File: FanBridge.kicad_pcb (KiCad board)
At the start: 2 copper layers, 15.2 x 10.2 mm, 15 parts, among them P1 CONN_01X01, P2 CONN_01X01, P3 CONN_1, P4 CONN_1, P5 CONN_1, P6 CONN_1, Q1 IRF7309IPBF, Q2 2N7002, Q3 2N7002, Q4 IRF7309IPBF

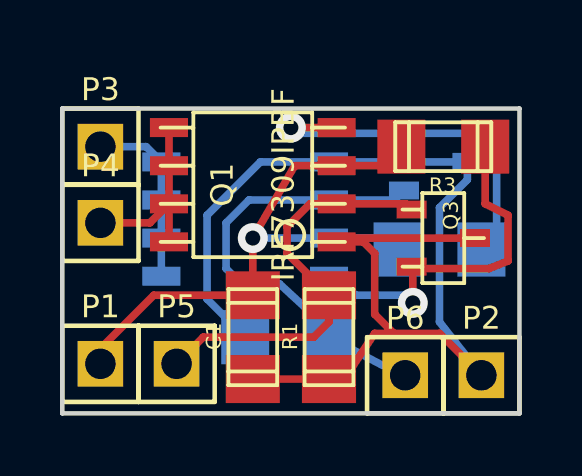
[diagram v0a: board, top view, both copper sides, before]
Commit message: 18.08.2017
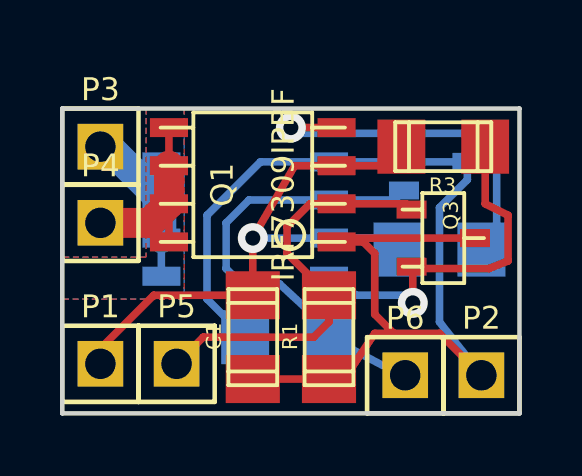
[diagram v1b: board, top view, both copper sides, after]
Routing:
- net /power+: track 6.36 -> 7.63 mm
- net /power-: track 6.05 -> 6.58 mm
- added copper zone on F.Cu, net /power+
- added copper zone on B.Cu, net /power-
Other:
- net class Output added: clearance 0.254, trace_width 1, via_dia 1, via_drill 0.635
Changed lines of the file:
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@@
     (thickness 1.6)
     (drawings 4)
-    (tracks 89)
+    (tracks 90)
     (zones 0)
     (modules 15)
@@
     (last_trace_width 0.254)
     (trace_clearance 0.254)
-    (zone_clearance 0.508)
+    (zone_clearance 0.5)
     (zone_45_only no)
     (trace_min 0.254)
@@
     (pad_to_mask_clearance 0.2)
     (aux_axis_origin 0 0)
-    (visible_elements FFFE5FBF)
+    (visible_elements FFFE7FBF)
     (pcbplotparams
       (layerselection 3178497)
@@
     (uvia_drill 0.127)
     (add_net "")
-    (add_net +8V)
     (add_net /control+)
     (add_net /control-)
+    (add_net N-000004)
+    (add_net N-000005)
+  )
+  (net_class Output ""
+    (clearance 0.254)
+    (trace_width 1)
+    (via_dia 1)
+    (via_drill 0.635)
+    (uvia_dia 0.508)
+    (uvia_drill 0.127)
     (add_net /power+)
     (add_net /power-)
-    (add_net GND)
-    (add_net N-000004)
-    (add_net N-000005)
   )
   (net_class Power ""
@@
     (uvia_dia 0.508)
     (uvia_drill 0.127)
+    (add_net +8V)
+    (add_net GND)
   )
   (module c_1206 (layer F.Cu)
@@
   (gr_line (start 121.92 73.66) (end 121.92 63.5) (angle 90) (layer Edge.Cuts) (width 0.15))
   (gr_line (start 137.16 73.66) (end 121.92 73.66) (angle 90) (layer Edge.Cuts) (width 0.15))
-  (segment (start 128.27 67.818) (end 128.27 69.723) (width 0.254) (layer F.Cu) (net 1) (status 800000))
-  (segment (start 123.19 72.009) (end 123.19 71.501) (width 0.254) (layer F.Cu) (net 1) (status C00000))
-  (segment (start 123.19 71.501) (end 124.968 69.723) (width 0.254) (layer F.Cu) (net 1) (status 400000))
-  (segment (start 124.968 69.723) (end 128.27 69.723) (width 0.254) (layer F.Cu) (net 1) (status 800000))
+  (segment (start 128.27 67.818) (end 128.27 69.723) (width 0.254) (layer F.Cu) (net 1))
+  (segment (start 123.19 72.009) (end 123.19 71.501) (width 0.254) (layer F.Cu) (net 1))
+  (segment (start 123.19 71.501) (end 124.968 69.723) (width 0.254) (layer F.Cu) (net 1))
+  (segment (start 124.968 69.723) (end 128.27 69.723) (width 0.254) (layer F.Cu) (net 1))
   (segment (start 128.27 67.818) (end 130.81 67.818) (width 0.254) (layer B.Cu) (net 1))
   (via (at 128.27 67.818) (size 1) (layers F.Cu B.Cu) (net 1))
@@
   (segment (start 133.223 72.39) (end 130.81 71.12) (width 0.254) (layer B.Cu) (net 2) (status 10))
   (segment (start 133.30936 66.2305) (end 133.24586 66.294) (width 0.254) (layer B.Cu) (net 2) (status 30))
-  (segment (start 131.064 66.675) (end 130.175 66.675) (width 0.254) (layer F.Cu) (net 3) (status 400000))
-  (segment (start 129.413 68.326) (end 130.81 69.723) (width 0.254) (layer F.Cu) (net 3) (status 800000))
+  (segment (start 131.064 66.675) (end 130.175 66.675) (width 0.254) (layer F.Cu) (net 3))
+  (segment (start 129.413 68.326) (end 130.81 69.723) (width 0.254) (layer F.Cu) (net 3))
   (segment (start 129.413 67.437) (end 129.413 68.326) (width 0.254) (layer F.Cu) (net 3))
   (segment (start 130.175 66.675) (end 129.413 67.437) (width 0.254) (layer F.Cu) (net 3))
-  (segment (start 125.73 72.009) (end 126.619 71.12) (width 0.254) (layer F.Cu) (net 3) (status 400000))
+  (segment (start 125.73 72.009) (end 126.619 71.12) (width 0.254) (layer F.Cu) (net 3))
   (segment (start 126.619 71.12) (end 130.302 71.12) (width 0.254) (layer F.Cu) (net 3))
   (segment (start 130.302 71.12) (end 130.81 70.612) (width 0.254) (layer F.Cu) (net 3))
-  (segment (start 130.81 70.612) (end 130.81 69.723) (width 0.254) (layer F.Cu) (net 3) (status 800000))
+  (segment (start 130.81 70.612) (end 130.81 69.723) (width 0.254) (layer F.Cu) (net 3))
   (segment (start 133.56336 66.8655) (end 133.37286 66.675) (width 0.254) (layer F.Cu) (net 3) (status 30))
   (segment (start 133.37286 66.675) (end 131.064 66.675) (width 0.254) (layer F.Cu) (net 3) (status 10))
-  (segment (start 123.19 67.31) (end 124.841 67.31) (width 0.254) (layer F.Cu) (net 4) (status 400000))
-  (segment (start 124.841 67.31) (end 125.476 66.675) (width 0.254) (layer F.Cu) (net 4) (status 800000))
-  (segment (start 125.476 64.135) (end 125.476 65.405) (width 0.254) (layer F.Cu) (net 4) (status C00000))
-  (segment (start 125.476 65.405) (end 125.476 66.675) (width 0.254) (layer F.Cu) (net 4) (status C00000))
-  (segment (start 125.476 66.675) (end 125.476 67.945) (width 0.254) (layer F.Cu) (net 4) (status C00000))
-  (segment (start 123.19 64.77) (end 124.714 64.77) (width 0.254) (layer B.Cu) (net 5) (status 400000))
-  (segment (start 124.714 64.77) (end 125.222 65.278) (width 0.254) (layer B.Cu) (net 5) (status 800000))
-  (segment (start 125.222 65.278) (end 125.222 66.548) (width 0.254) (layer B.Cu) (net 5) (status C00000))
-  (segment (start 125.222 66.548) (end 125.222 67.818) (width 0.254) (layer B.Cu) (net 5) (status C00000))
-  (segment (start 125.222 67.818) (end 125.222 69.088) (width 0.254) (layer B.Cu) (net 5) (status C00000))
-  (segment (start 130.81 72.517) (end 128.27 72.517) (width 0.254) (layer F.Cu) (net 6) (status C00000))
+  (segment (start 123.19 67.31) (end 124.841 67.31) (width 1) (layer F.Cu) (net 4) (status 400000))
+  (segment (start 124.841 67.31) (end 125.476 66.675) (width 1) (layer F.Cu) (net 4) (status 800000))
+  (segment (start 125.476 66.675) (end 125.476 65.405) (width 1) (layer F.Cu) (net 4) (status C00000))
+  (segment (start 125.476 64.135) (end 125.476 65.405) (width 0.254) (layer F.Cu) (net 4))
+  (segment (start 125.476 65.405) (end 125.476 66.675) (width 0.254) (layer F.Cu) (net 4))
+  (segment (start 125.476 66.675) (end 125.476 67.945) (width 0.254) (layer F.Cu) (net 4))
+  (segment (start 125.222 67.818) (end 125.222 66.548) (width 1) (layer B.Cu) (net 5) (status C00000))
+  (segment (start 123.19 64.77) (end 123.444 64.77) (width 1) (layer B.Cu) (net 5) (status C00000))
+  (segment (start 123.444 64.77) (end 125.222 66.548) (width 1) (layer B.Cu) (net 5) (status C00000))
+  (segment (start 125.222 65.278) (end 125.222 66.548) (width 0.254) (layer B.Cu) (net 5))
+  (segment (start 125.222 67.818) (end 125.222 69.088) (width 0.254) (layer B.Cu) (net 5))
+  (segment (start 130.81 72.517) (end 128.27 72.517) (width 0.254) (layer F.Cu) (net 6))
   (segment (start 132.969 70.993) (end 132.334 70.993) (width 0.254) (layer F.Cu) (net 6))
   (segment (start 132.334 70.993) (end 131.318 72.517) (width 0.254) (layer F.Cu) (net 6) (status 20))
@@
   (segment (start 136.0805 64.3255) (end 136.398 64.643) (width 0.254) (layer B.Cu) (net 8))
   (zone (net 1) (net_name +8V) (layer F.Cu) (hatch full 0.508)
+    (connect_pads (clearance 0.75))
+    (min_thickness 0.254)
+    (fill (arc_segments 16) (thermal_gap 0.508) (thermal_bridge_width 0.508))
+    (polygon
+      (pts
+        (xy 125.984 63.881) (xy 125.984 69.85) (xy 121.92 69.85) (xy 121.92 73.66) (xy 137.16 73.66)
+        (xy 137.16 63.5) (xy 125.984 63.5)
+      )
+    )
+  )
+  (zone (net 6) (net_name GND) (layer B.Cu) (hatch edge 0.508)
+    (connect_pads (clearance 0.75))
+    (min_thickness 0.254)
+    (fill (arc_segments 16) (thermal_gap 0.508) (thermal_bridge_width 0.508))
+    (polygon
+      (pts
+        (xy 125.984 64.643) (xy 125.984 69.85) (xy 121.92 69.85) (xy 121.92 73.66) (xy 137.16 73.66)
+        (xy 137.16 63.5) (xy 125.984 63.5)
+      )
+    )
+  )
+  (zone (net 5) (net_name /power-) (layer B.Cu) (hatch edge 0.508)
+    (connect_pads (clearance 0.5))
+    (min_thickness 0.254)
+    (fill (arc_segments 16) (thermal_gap 0.508) (thermal_bridge_width 0.508))
+    (polygon
+      (pts
+        (xy 121.92 63.5) (xy 124.714 63.5) (xy 124.714 68.453) (xy 121.92 68.453)
+      )
+    )
+  )
+  (zone (net 4) (net_name /power+) (layer F.Cu) (hatch edge 0.508)
     (connect_pads (clearance 1))
     (min_thickness 0.254)
@@
     (polygon
       (pts
-        (xy 121.92 63.5) (xy 121.92 73.66) (xy 137.16 73.66) (xy 137.16 63.5)
+        (xy 121.92 63.5) (xy 124.714 63.5) (xy 124.714 68.453) (xy 121.92 68.453)
       )
     )
-  )
-  (zone (net 6) (net_name GND) (layer B.Cu) (hatch edge 0.508)
-    (connect_pads (clearance 1))
-    (min_thickness 0.254)
-    (fill (arc_segments 16) (thermal_gap 0.508) (thermal_bridge_width 0.508))
-    (polygon
-      (pts
-        (xy 121.92 63.5) (xy 121.92 73.66) (xy 137.16 73.66) (xy 137.16 63.5)
-      )
-    )
